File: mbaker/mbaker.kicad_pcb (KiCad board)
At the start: 4 copper layers, 75 x 10 mm, 21 parts, among them J1 AVR ISP, U1 ATTINY84A-SSFR, U2 RN4871, U3 FM24V10, U4 ICM-20602, U5 MCP130-270TT, Y1 ABM10W-20.0000MHZ-8-D1X-T3

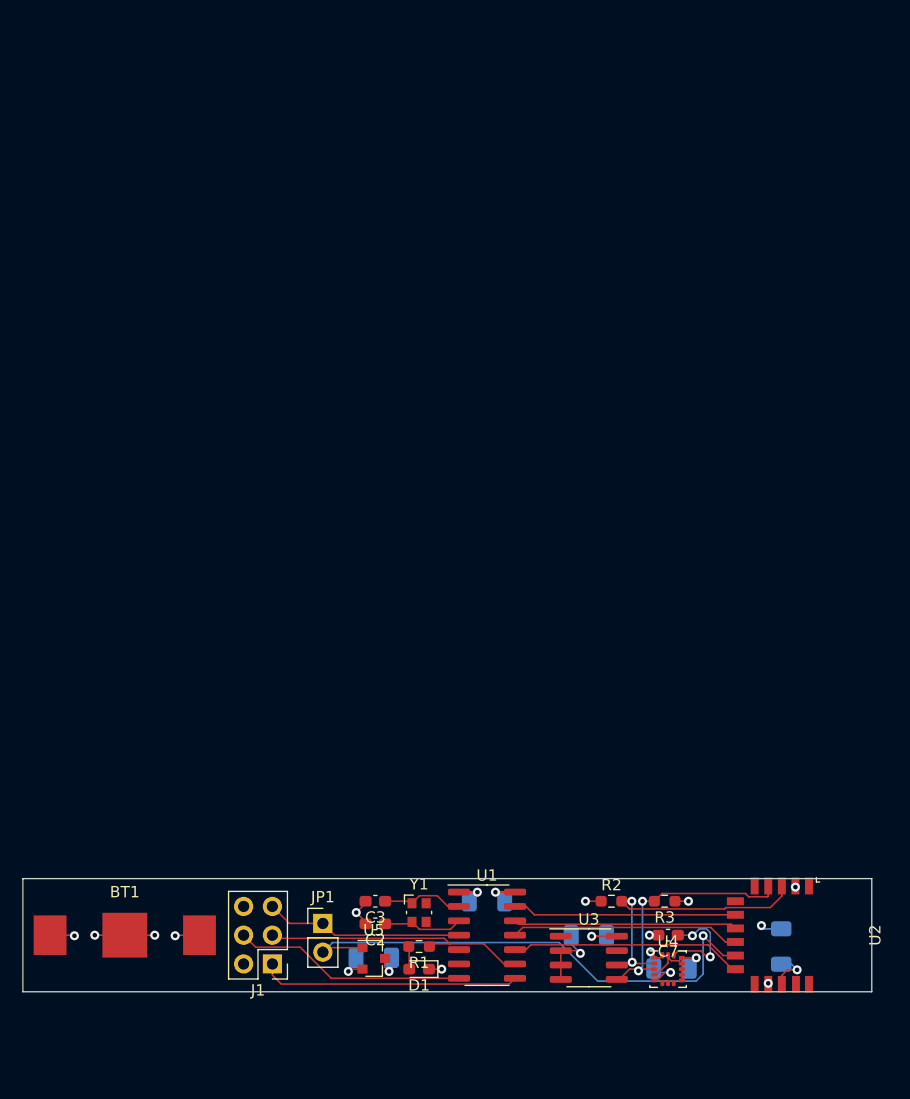
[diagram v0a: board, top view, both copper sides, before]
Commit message: Finalized 2.3.1 prototype
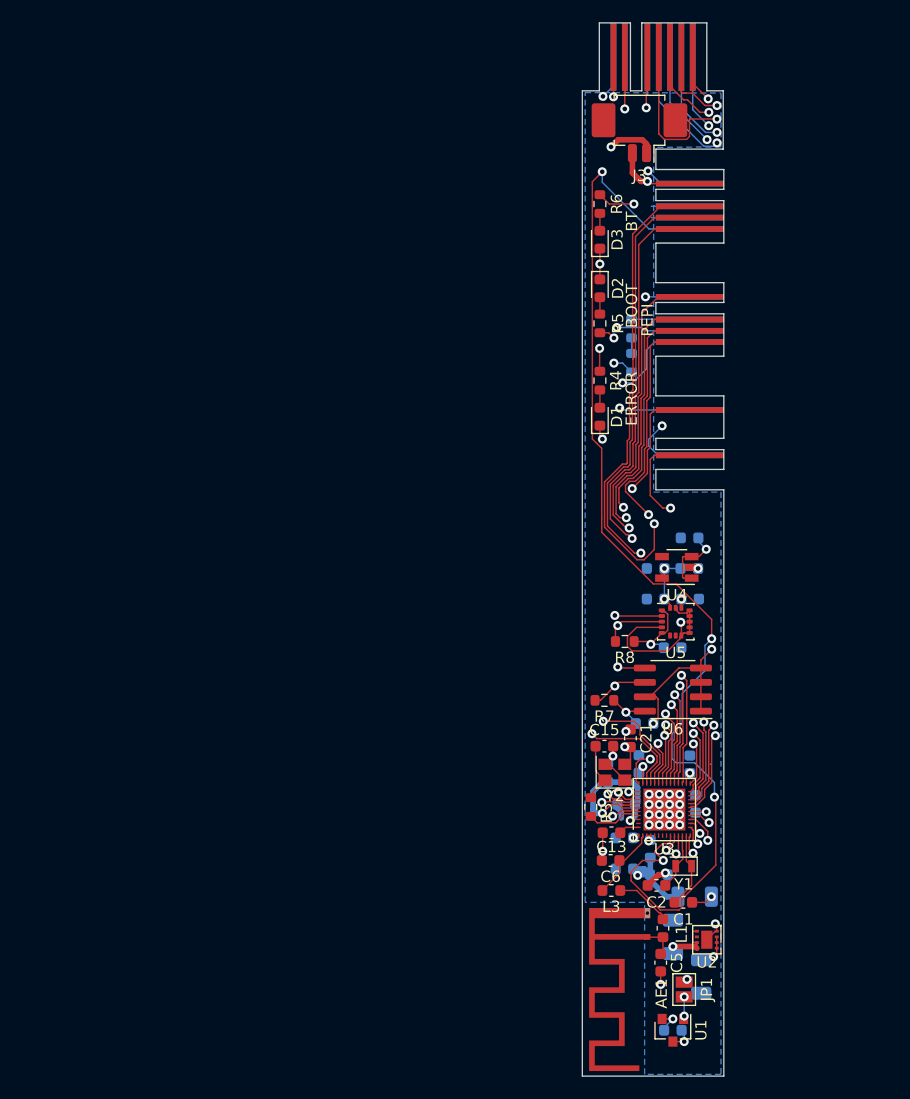
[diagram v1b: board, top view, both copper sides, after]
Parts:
- removed BT1: 1025 Lithium Battery, mbaker:3030_1x1025
- added AE1: PCB Antenna, RF_Antenna:Texas_SWRA117D_2.4GHz_Left, F.Cu at (150.2, 135.2)
- added C10: 10uF, Capacitor_SMD:C_1206_3216Metric, B.Cu at (154.3, 131.6)
- added C11: 1uF, Capacitor_SMD:C_0603_1608Metric, B.Cu at (153.9, 99.9)
- added C12: 1uF, Capacitor_SMD:C_0603_1608Metric, B.Cu at (153.9, 119.9)
- added C13: 10nF, Capacitor_SMD:C_0603_1608Metric, F.Cu at (147.0, 126.0)
- added C14: 1uF, Capacitor_SMD:C_0603_1608Metric, B.Cu at (153.9, 102.6)
- added C15: 12pF, Capacitor_SMD:C_0603_1608Metric, F.Cu at (146.4, 118.3)
- added C16: 100nF, Capacitor_SMD:C_0603_1608Metric, B.Cu at (154.4, 123.4)
- added C17: 100nF, Capacitor_SMD:C_0603_1608Metric, B.Cu at (149.4, 119.9)
- added C18: 100nF, Capacitor_SMD:C_0603_1608Metric, B.Cu at (148.2, 126.4)
- added C19: 1uF, Capacitor_SMD:C_0603_1608Metric, B.Cu at (146.7, 120.7)
- added C20: 100pF, Capacitor_SMD:C_0603_1608Metric, B.Cu at (148.3, 123.5)
- added C21: 12pF, Capacitor_SMD:C_0603_1608Metric, F.Cu at (148.7, 117.6)
- added C22: 2.2uF, Capacitor_SMD:C_0603_1608Metric, B.Cu at (150.9, 102.6)
- added C23: 100nF, Capacitor_SMD:C_0603_1608Metric, B.Cu at (150.9, 105.3)
- added C24: 10nF, Capacitor_SMD:C_0603_1608Metric, B.Cu at (152.4, 109.6)
- added C25: 2.2uF, Capacitor_SMD:C_0603_1608Metric, B.Cu at (149.9, 116.3)
- added C26: 470nF, Capacitor_SMD:C_0603_1608Metric, B.Cu at (153.9, 105.3)
- added C9: 100nF, Capacitor_SMD:C_0603_1608Metric, B.Cu at (148.2, 129.2)
- added D2: 2.1V, Diode_SMD:D_0603_1608Metric, F.Cu at (146.0, 77.8)
- added D3: 2.1V, Diode_SMD:D_0603_1608Metric, F.Cu at (146.0, 73.5)
- added J2: PEGI, mbaker:PEGI, F.Cu at (157.0, 53.4)
- added J3: 53261-7002, Connector_Molex:Molex_PicoBlade_53261-0271_1x02-1MP_P1.25mm_Horizontal, F.Cu at (149.5, 63.5)
- added L1: L, Inductor_SMD:L_0603_1608Metric, F.Cu at (151.6, 134.4)
- added L2: 2nH, Inductor_SMD:L_0603_1608Metric, B.Cu at (150.4, 127.4)
- added L3: L, Inductor_SMD:L_0603_1608Metric, F.Cu at (147.0, 131.1)
- added R4: 120Ω, Resistor_SMD:R_0603_1608Metric, F.Cu at (146.0, 86.0)
- added R5: 120Ω, Resistor_SMD:R_0603_1608Metric, F.Cu at (146.0, 81.0)
- added R6: 120Ω, Resistor_SMD:R_0603_1608Metric, F.Cu at (146.0, 70.4)
- added R7: 12kΩ, Resistor_SMD:R_0603_1608Metric, F.Cu at (146.4, 114.2)
- added R8: 12kΩ, Resistor_SMD:R_0603_1608Metric, F.Cu at (148.2, 109.0)
- added U6: FM24V01, Package_SO:SOIC-8_3.9x4.9mm_P1.27mm, F.Cu at (152.4, 113.3)
- added Y2: 40MHZ, Crystal:Crystal_SMD_2520-4Pin_2.5x2.0mm, F.Cu at (147.3, 120.6)
- C1: value 10uF -> 12pF; footprint Capacitor_SMD:C_1206_3216Metric_Pad1.33x1.80mm_HandSolder -> Capacitor_SMD:C_0603_1608Metric; moved to F.Cu
- C2: value 18pF -> 12pF; footprint Capacitor_SMD:C_0603_1608Metric_Pad1.08x0.95mm_HandSolder -> Capacitor_SMD:C_0603_1608Metric
- C3: value 18pF -> 100nF; footprint Capacitor_SMD:C_0603_1608Metric_Pad1.08x0.95mm_HandSolder -> Capacitor_SMD:C_0603_1608Metric; moved to B.Cu
- C4: footprint Capacitor_SMD:C_1206_3216Metric_Pad1.33x1.80mm_HandSolder -> Capacitor_SMD:C_1206_3216Metric
- C5, C6: value 10uF -> C; footprint Capacitor_SMD:C_1206_3216Metric_Pad1.33x1.80mm_HandSolder -> Capacitor_SMD:C_0603_1608Metric; moved to F.Cu
- C7: value 0.1uF -> 10uF; footprint Capacitor_SMD:C_0603_1608Metric_Pad1.08x0.95mm_HandSolder -> Capacitor_SMD:C_1206_3216Metric; moved to B.Cu
- C8: value 10uF -> 1uF; footprint Capacitor_SMD:C_1206_3216Metric_Pad1.33x1.80mm_HandSolder -> Capacitor_SMD:C_0603_1608Metric
- D1: value LTST-C193TBKT-5A -> 2.1V; footprint LED_SMD:LED_0603_1608Metric_Pad1.05x0.95mm_HandSolder -> Diode_SMD:D_0603_1608Metric
- J1: value AVR ISP -> PEPI; footprint Connector_PinHeader_2.54mm:PinHeader_2x03_P2.54mm_Vertical -> mbaker:PEPI
- JP1: value Programming Disconnect -> Reset Disconnect; footprint Connector_PinHeader_2.54mm:PinHeader_1x02_P2.54mm_Vertical -> Jumper:SolderJumper-2_P1.3mm_Open_Pad1.0x1.5mm
- R1: value 330ohm -> 22Ω; footprint Resistor_SMD:R_0603_1608Metric_Pad0.98x0.95mm_HandSolder -> Resistor_SMD:R_0603_1608Metric; moved to B.Cu
- R2: value 10kOhm -> 470Ω; footprint Resistor_SMD:R_0603_1608Metric_Pad0.98x0.95mm_HandSolder -> Resistor_SMD:R_0603_1608Metric; moved to B.Cu
- R3: value 10kOhm -> 0Ω; footprint Resistor_SMD:R_0603_1608Metric_Pad0.98x0.95mm_HandSolder -> Resistor_SMD:R_0603_1608Metric
- U1: value ATTINY84A-SSFR -> MCP130T-270I/TT; footprint Package_SO:SOIC-14_3.9x8.7mm_P1.27mm -> Package_TO_SOT_SMD:SOT-23
- U2: value RN4871 -> ADP124ACPZ-3.3-R7; footprint RF_Module:Microchip_RN4871 -> mbaker:LFCSP-8_2x2mm_0.5pitch
- U3: value FM24V10 -> ESP32-U4WDH; footprint Package_SO:SOIC-8_3.9x4.9mm_P1.27mm -> mbaker:QFN48_5x5mm_1EP
- U4: value ICM-20602 -> ADP150AUJZ-1.8-R7; footprint Package_LGA:LGA-16_3x3mm_P0.5mm_LayoutBorder3x5y -> Package_TO_SOT_SMD:TSOT-23-5
- U5: value MCP130-270TT -> ICM-20601; footprint Package_TO_SOT_SMD:SOT-23 -> Package_LGA:LGA-16_3x3mm_P0.5mm_LayoutBorder3x5y
- Y1: value ABM10W-20.0000MHZ-8-D1X-T3 -> 32.768kHZ; footprint Crystal:Crystal_SMD_Abracon_ABM10-4Pin_2.5x2.0mm -> Crystal:Crystal_SMD_2012-2Pin_2.0x1.2mm
- moved J1 58.7 mm to (157.9, 95.4), turned to 90 degrees
- moved R1 57.7 mm to (148.8, 81.4), turned to 90 degrees
- moved D1 51.4 mm to (146.0, 89.2), turned to 90 degrees
- moved R2 47.6 mm to (148.8, 84.4), turned to 90 degrees
- moved U5 40.0 mm to (152.7, 107.3)
- moved U4 35.5 mm to (152.8, 102.5), turned to 180 degrees
- moved JP1 32.5 mm to (153.4, 139.8), turned to 90 degrees
- moved C3 28.7 mm to (152.4, 143.4), turned to 0 degrees
- moved C8 26.2 mm to (151.2, 129.7)
- moved C2 25.1 mm to (151.0, 130.6)
- moved Y1 23.7 mm to (153.4, 128.9), turned to 180 degrees
- moved U1 18.4 mm to (152.4, 143.4), turned to 270 degrees
- moved C1 17.4 mm to (153.3, 132.1)
- moved U3 11.4 mm to (149.2, 126.4)
- moved C6 11.0 mm to (146.9, 128.4), turned to 180 degrees
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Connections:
- C1 pad 1: +BATT -> Net-(C1-Pad1)
- C3 pad 1: Net-(C3-Pad1) -> +3V3
- C4 pad 1: +BATT -> Net-(C4-Pad1)
- C5 pad 1: +BATT -> Net-(AE1-Pad1)
- C6 pad 1: +BATT -> Net-(C6-Pad1)
- C7 pad 1: Net-(C7-Pad1) -> +3V3
- C8 pad 1: +BATT -> +3V3
- J1 pad 1: Net-(J1-Pad1) -> Earth
- J1 pad 2: +BATT -> SPI_CS
- J1 pad 3: Net-(J1-Pad3) -> SPI_IO1
- J1 pad 4: Net-(J1-Pad4) -> SPI_IO3
- J1 pad 5: Net-(J1-Pad5) -> SPI_CLK
- J1 pad 6: Earth -> SPI_IO2
- JP1 pad 1: Net-(J1-Pad5) -> Net-(JP1-Pad1)
- R1 pad 1: Net-(J1-Pad3) -> Net-(R1-Pad1)
- R1 pad 2: Net-(D1-Pad2) -> UART_TX
- R2 pad 1: +BATT -> Net-(R2-Pad1)
- R2 pad 2: Net-(R2-Pad2) -> Net-(R1-Pad1)
- R3 pad 1: +BATT -> Net-(R3-Pad1)
- R3 pad 2: Net-(R3-Pad2) -> Net-(C15-Pad1)
- U1 pad 1: +BATT -> Net-(JP1-Pad1)
- U1 pad 2: Net-(C3-Pad1) -> +3V3
- U1 pad 3: Net-(C2-Pad1) -> Earth
- U2 pad 1: Net-(U2-Pad1) -> +3V3
- U2 pad 2: Earth -> +3V3
- U2 pad 3: Net-(R2-Pad2) -> +3V3
- U2 pad 4: Net-(R3-Pad2) -> Earth
- U2 pad 5: Net-(U2-Pad5) -> Net-(C4-Pad1)
- U2 pad 6: Net-(U2-Pad6) -> (no net)
- U2 pad 7: Net-(U1-Pad13) -> Net-(C4-Pad1)
- U2 pad 8: Net-(U1-Pad12) -> Net-(C4-Pad1)
- U3 pad 1: Net-(U3-Pad1) -> +3V3
- U3 pad 2: Earth -> Net-(C6-Pad1)
- U3 pad 3: Earth -> Net-(L2-Pad2)
- U3 pad 4: Earth -> Net-(L2-Pad2)
- U3 pad 5: Net-(R3-Pad2) -> Net-(U3-Pad5)
- U3 pad 6: Net-(R2-Pad2) -> Net-(U3-Pad6)
- U3 pad 8: +BATT -> Net-(U3-Pad8)
- U4 pad 1: +BATT -> +3V3
- U4 pad 2: Net-(R2-Pad2) -> Earth
- U4 pad 3: Net-(R3-Pad2) -> +3V3
- U4 pad 4: Earth -> (no net)
- U4 pad 5: +BATT -> +1V8
- U5 pad 1: RESET -> +3V3
- U5 pad 2: +BATT -> I2C_SCK
- U5 pad 3: Earth -> I2C_SDA
- Y1 pad 1: Net-(C3-Pad1) -> Net-(C1-Pad1)
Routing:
- net Net-(C4-Pad1): track 0.00 -> 86.7 mm, vias 0 -> 2
- net GPIO27: track 0.00 -> 84.1 mm, vias 0 -> 2
- net GPIO34: track 0.00 -> 83.9 mm, vias 0 -> 2
- net GPIO10: track 0.00 -> 83.8 mm, vias 0 -> 2
- net GPIO2: track 0.00 -> 81.5 mm, vias 0 -> 2
- net GPIO35: track 0.00 -> 79.8 mm, vias 0 -> 2
- net GPIO22: track 0.00 -> 79.2 mm, vias 0 -> 2
- net GPIO21: track 0.00 -> 78.6 mm, vias 0 -> 2
- net GPIO4: track 0.00 -> 77.5 mm, vias 0 -> 2
- net GPIO19: track 0.00 -> 77.3 mm, vias 0 -> 2
- net GPIO9: track 0.00 -> 76.2 mm, vias 0 -> 2
- net SPI_CS: track 0.00 -> 68.4 mm, vias 0 -> 2
- net I2C_SDA: track 0.00 -> 66.7 mm, vias 0 -> 4
- net RESET: track 46.2 -> 112.0 mm, vias 1 -> 5
- net I2C_SCK: track 0.00 -> 61.0 mm, vias 0 -> 4
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- added copper zone on In1.Cu, net +3V3
- added copper zone on B.Cu, net Earth
- removed copper zone on In1.Cu, net +BATT
- removed copper zone on In2.Cu, net Earth
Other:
- board size 75 x 10 mm -> 12.5 x 93 mm
- net class Default: clearance 0.14 -> 0.127; trace_width 0.14 -> 0.127
- net class Power added: clearance 0.127, trace_width 0.5, via_dia 0.8, via_drill 0.4
- rule trace_clearance: 0.14 -> 0.127
- rule trace_min: 0.14 -> 0.127
- board text added: "BOOT"
- board text added: "BT"
- board text added: "ERROR"
